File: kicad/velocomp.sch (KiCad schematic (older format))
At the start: 32 parts, among them IC1 STM8S003F3P, J1 USB_B, J2 h2_g, J3 prg, J4 h2, J5 kn1, J6 kn1, J7 ind, J8 ind, Q1 2N7002, SW1 SW_PUSH, SW2 Herkon, U1 BK3231, U2 TP4056, Y1 8Mgh

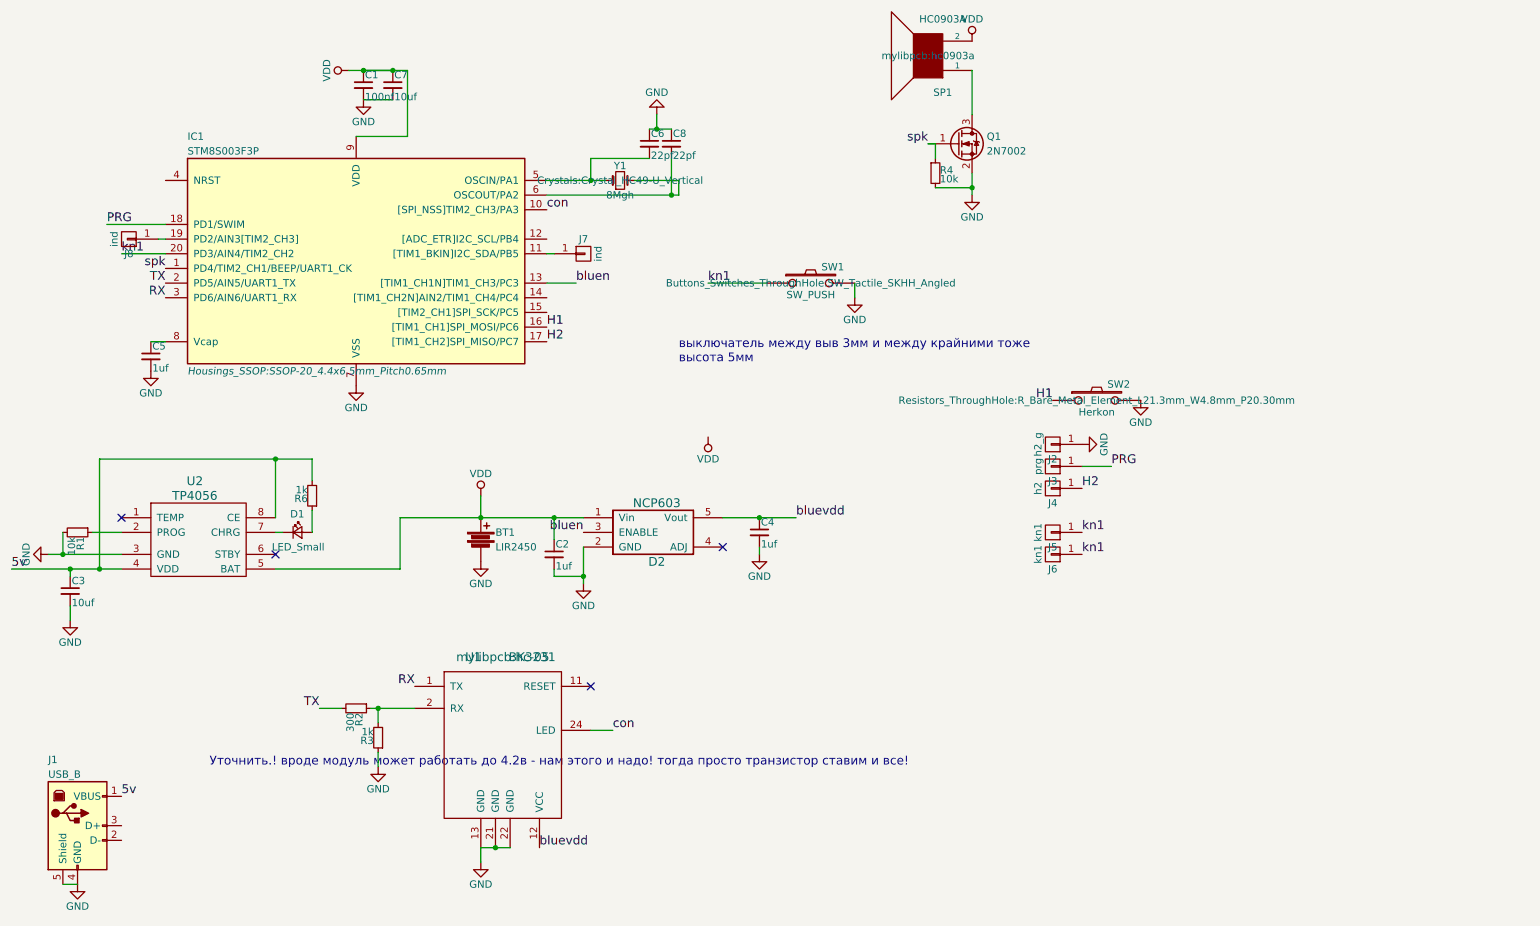
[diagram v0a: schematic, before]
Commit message: start
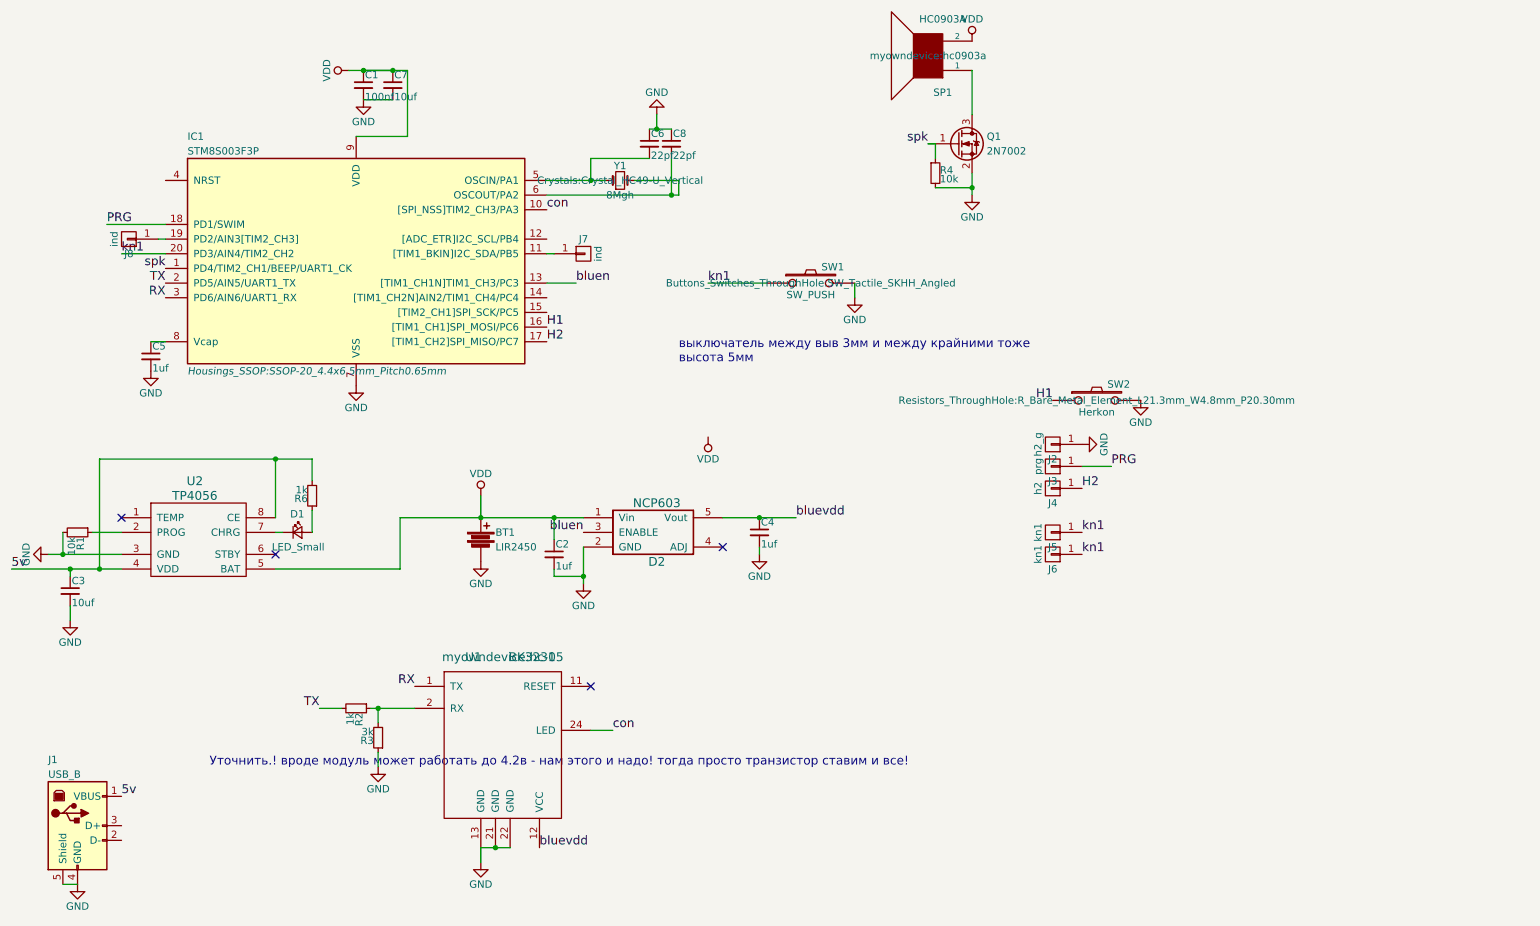
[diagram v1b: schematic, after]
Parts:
- J1: footprint mylibpcb:usb5s -> myowndevice:usb5s
- R2: value 300 -> 1k
- R3: value 1k -> 3k
- SP1: footprint mylibpcb:hc0903a -> myowndevice:hc0903a
- U1: footprint mylibpcb:hc-05 -> myowndevice:hc-05
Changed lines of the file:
@@
 F 0 "U1" H 4300 5200 60  0000 C CNN
 F 1 "BK3231" H 4700 5200 60  0000 C CNN
-F 2 "mylibpcb:hc-05" H 4500 5200 60  0000 C CNN
+F 2 "myowndevice:hc-05" H 4500 5200 60  0000 C CNN
 F 3 "" H 4500 5200 60  0000 C CNN
 	1    4500 5200
@@
 F 0 "SP1" H 7300 1350 50  0000 C CNN
 F 1 "HC0903A" H 7300 850 50  0000 C CNN
-F 2 "mylibpcb:hc0903a" H 7400 1100 50  0000 C CNN
+F 2 "myowndevice:hc0903a" H 7400 1100 50  0000 C CNN
 F 3 "" H 7400 1100 50  0000 C CNN
 	1    7400 1100
@@
 F 0 "J1" H 1400 6800 50  0000 L CNN
 F 1 "USB_B" H 1400 6700 50  0000 L CNN
-F 2 "mylibpcb:usb5s" H 1750 6300 50  0001 C CNN
+F 2 "myowndevice:usb5s" H 1750 6300 50  0001 C CNN
 F 3 "" H 1750 6300 50  0001 C CNN
 	1    1600 6350
@@
 P 3500 5550
 F 0 "R2" H 3530 5570 50  0000 L CNN
-F 1 "300" H 3530 5510 50  0000 L CNN
+F 1 "1k" H 3530 5510 50  0000 L CNN
 F 2 "Resistors_SMD:R_0603_HandSoldering" H 3500 5550 50  0001 C CNN
 F 3 "" H 3500 5550 50  0001 C CNN
@@
 P 3650 5750
 F 0 "R3" H 3680 5770 50  0000 L CNN
-F 1 "1k" H 3680 5710 50  0000 L CNN
+F 1 "3k" H 3680 5710 50  0000 L CNN
 F 2 "Resistors_SMD:R_0603_HandSoldering" H 3650 5750 50  0001 C CNN
 F 3 "" H 3650 5750 50  0001 C CNN
